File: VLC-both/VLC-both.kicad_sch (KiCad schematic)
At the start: 8 parts, among them J1 40HAT, J3 40HAT, U1 MCP3008

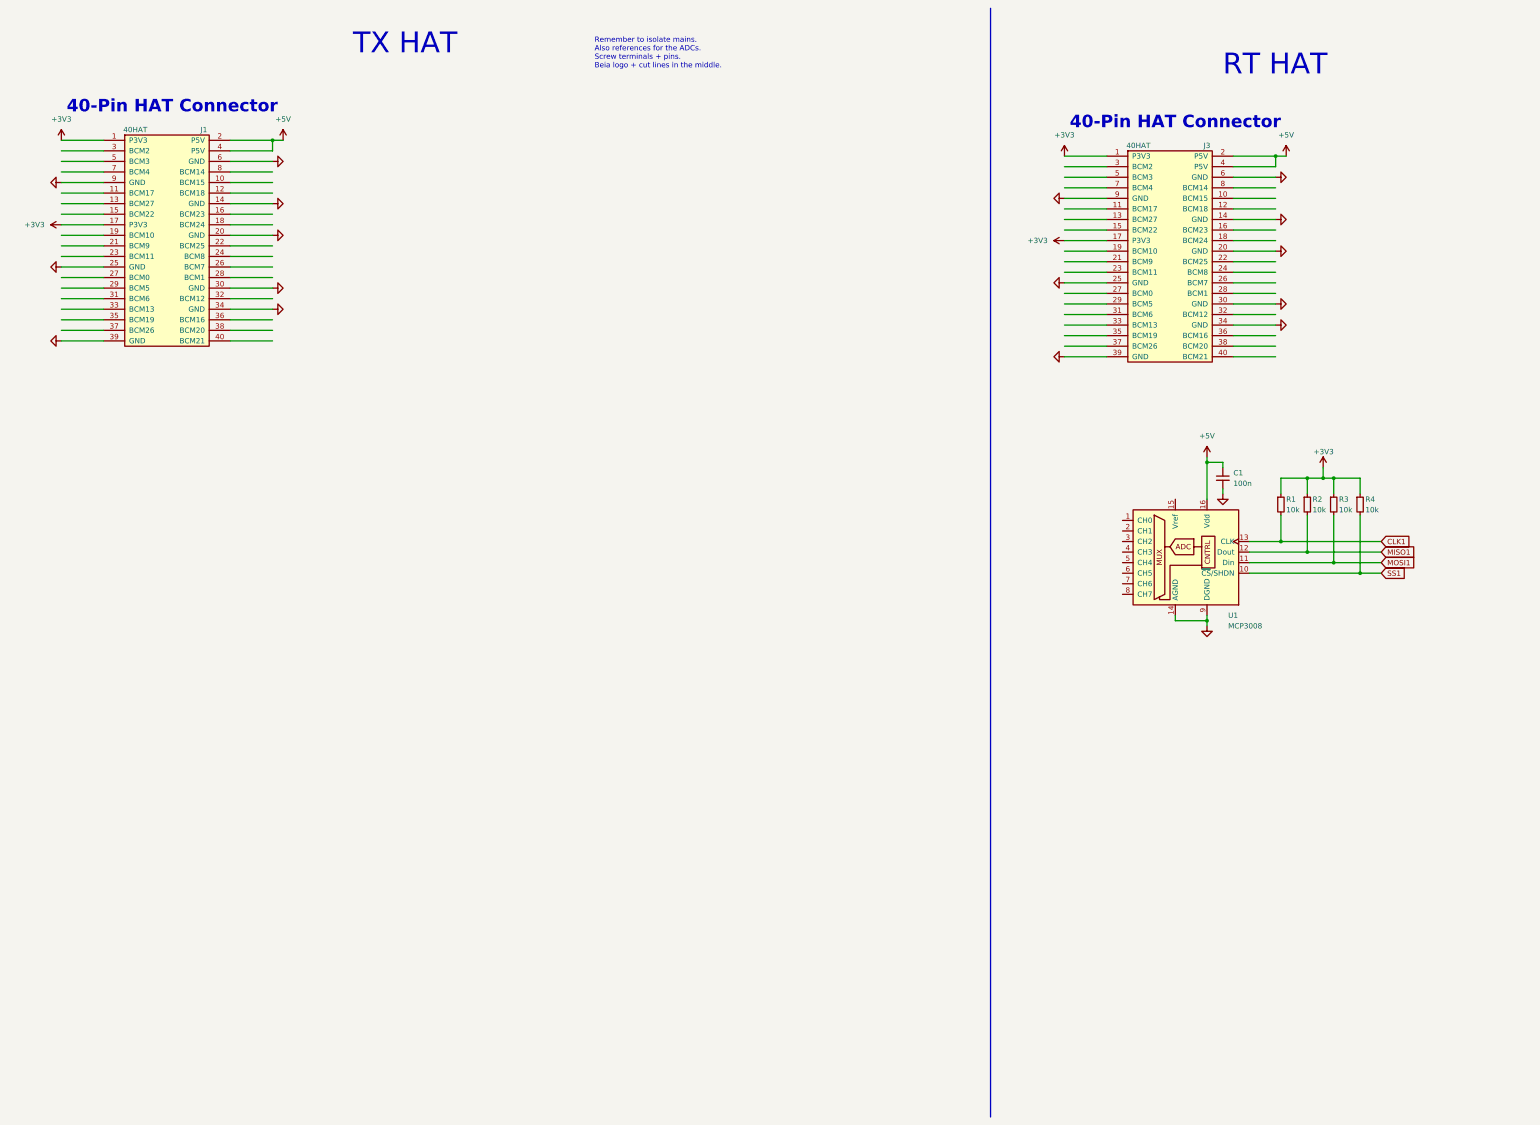
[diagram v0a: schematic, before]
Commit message: c
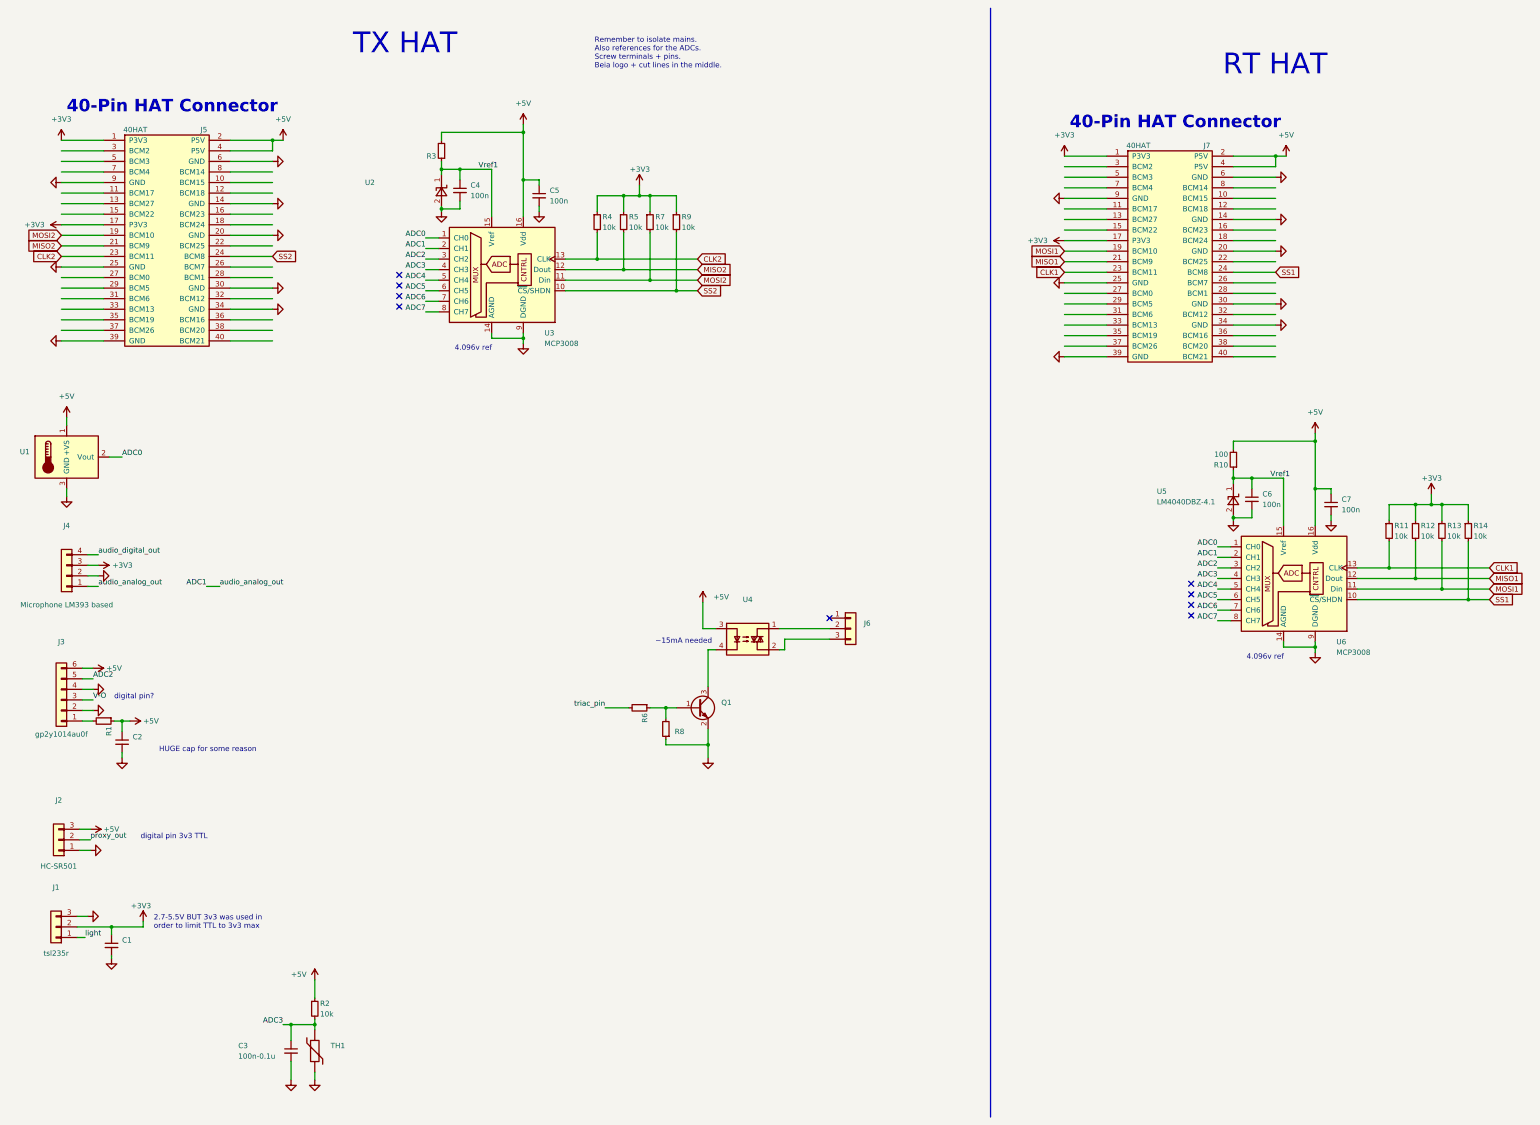
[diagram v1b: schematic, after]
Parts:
- removed U1: MCP3008, Package_SO:SOIC-16_3.9x9.9mm_P1.27mm, symbol Analog_ADC:MCP3008
- added C2: (no value), symbol Device:C_Small
- added C3: 100n-0.1u, Capacitor_SMD:C_0805_2012Metric, symbol Device:C_Small
- added C4, C5, C6, C7: 100n, Capacitor_SMD:C_0805_2012Metric, symbol Device:C_Small
- added J1, J2, J6: (no value), symbol Connector_Generic:Conn_01x03
- added J3: (no value), symbol Connector_Generic:Conn_01x06
- added J4: (no value), symbol Connector_Generic:Conn_01x04
- added Q1: (no value), symbol Device:Q_NPN_BEC
- added R10: 100, Resistor_SMD:R_0805_2012Metric, symbol Device:R_Small
- added R11, R12, R13, R14, R5, R7, R9: 10k, Resistor_SMD:R_0805_2012Metric, symbol Device:R_Small
- added R6, R8: (no value), symbol Device:R_Small
- added TH1: (no value), symbol Device:Thermistor
- added U1: (no value), symbol Sensor_Temperature:LM35-LP
- added U2: (no value), symbol Reference_Voltage:LM4040DBZ-4.1
- added U3, U6: MCP3008, Package_SO:SOIC-16_3.9x9.9mm_P1.27mm, symbol Analog_ADC:MCP3008
- added U4: (no value), symbol Relay_SolidState:S102S01
- added U5: LM4040DBZ-4.1, Package_TO_SOT_SMD:SOT-23, symbol Reference_Voltage:LM4040DBZ-4.1
- C1: value 100n -> (none); footprint Capacitor_SMD:C_0805_2012Metric -> (none)
- R1, R3: value 10k -> (none); footprint Resistor_SMD:R_0805_2012Metric -> (none)
- renumbered J1 to J5, J3 to J7
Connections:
- net +3V3: now also C1.1, J1.2 (Pin_2), J4.3 (Pin_3), R11.1, R12.1, R13.1, R14.1, R5.1, R7.1, R9.1; no longer R1.1, R2.1, R3.1
- net +5V: now also R1.1, R2.1, R3.2, C2.1, C5.1, C7.1, J2.3 (Pin_3), J3.6 (Pin_6), R10.2, U1.1 (+VS), U3.16 (Vdd), U4.3, U6.16 (Vdd); no longer C1.1
- net CLK1: now also J7.23 (BCM11), R11.2, U6.13 (CLK); no longer R1.2
- net GND: now also C2.2, C3.2, C4.2, C5.2, C6.2, C7.2, J1.3 (Pin_3), J2.1 (Pin_1), J3.2 (Pin_2), J3.4 (Pin_4), J4.2 (Pin_2), Q1.2 (E), R8.1, TH1.2, U1.3 (GND), U2.2 (A), U3.14 (AGND), U3.9 (DGND), U5.2 (A), U6.14 (AGND), U6.9 (DGND)
- net MISO1: now also J7.21 (BCM9), R12.2, U6.12 (Dout); no longer R2.2
- net MOSI1: now also J7.19 (BCM10), R13.2, U6.11 (Din); no longer R3.2
- net SS1: now also J7.24 (BCM8), R14.2, U6.10 (~{CS}/SHDN); no longer R4.2
- net MOSI2: now reaches J5.19 (BCM10)
- net MOSI2: now also R7.2, U3.11 (Din)
- net MISO2: now reaches J5.21 (BCM9)
- net MISO2: now also R5.2, U3.12 (Dout)
- net CLK2: now reaches J5.23 (BCM11)
- net CLK2: now also R4.2, U3.13 (CLK)
- net SS2: now reaches J5.24 (BCM8)
- net SS2: now also R9.2, U3.10 (~{CS}/SHDN)
- new net: J3.1 (Pin_1), R1.2
- new net: J6.2 (Pin_2), U4.1
- new net: J6.3 (Pin_3), U4.2
- new net: Q1.1 (B), R6.1, R8.2
- new net: Q1.3 (C), U4.4
- new net ADC0: U1.2 (Vout), U3.1 (CH0), U6.1 (CH0)
- new net ADC1: J4.1 (Pin_1), U3.2 (CH1), U6.2 (CH1)
- new net ADC2: J3.5 (Pin_5), U3.3 (CH2), U6.3 (CH2)
- new net ADC3: C3.1, R2.2, TH1.1, U3.4 (CH3), U6.4 (CH3)
- new net ADC4: U3.5 (CH4), U6.5 (CH4)
- new net ADC5: U3.6 (CH5), U6.6 (CH5)
- new net ADC6: U3.7 (CH6), U6.7 (CH6)
- new net ADC7: U3.8 (CH7), U6.8 (CH7)
- new net V-O: J3.3 (Pin_3)
- new net Vref1: C4.1, C6.1, R10.1, R3.1, U2.1 (K), U3.15 (Vref), U5.1 (K), U6.15 (Vref)
- new net audio_digital_out: J4.4 (Pin_4)
- new net light: J1.1 (Pin_1)
- new net proxy_out: J2.2 (Pin_2)
- new net triac_pin: R6.2
- no-connect marks 0 -> 9
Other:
- note added: "2.7-5.5V BUT 3v3 was used in order to limit TTL to 3v3 max"
- note added: "4.096v ref"
- note added: "HUGE cap for some reason"
- note added: "digital pin 3v3 TTL"
- note added: "digital pin?"
- note added: "~15mA needed"
